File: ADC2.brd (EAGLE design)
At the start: 99.1 x 88.9 mm, 166 parts, among them IC1 FPGA CORE BOARD, IC10 AK1110, IC11 AD4001, IC12 TAR5SB33, IC13 74HC3G34, IC14 TC7WH74FU, IC15 NJM12888F18, IC16 TAR5SB33, IC2 OPA, IC3 OPA-DIFF, IC4 DCDC2, IC5 OPA-DIFF, IC6 OPA-DIFF, IC7 LM317-L, IC8 LM337-L, IC9 LM337-L, J1 DC, J10 ADC+, J11 GND, J12 ADC-, J2 DC, J3 VCOM, J4 GND, J5 VCOM, J6 V-, J7 V-, J8 V-, J9 V-, X1 12MHz

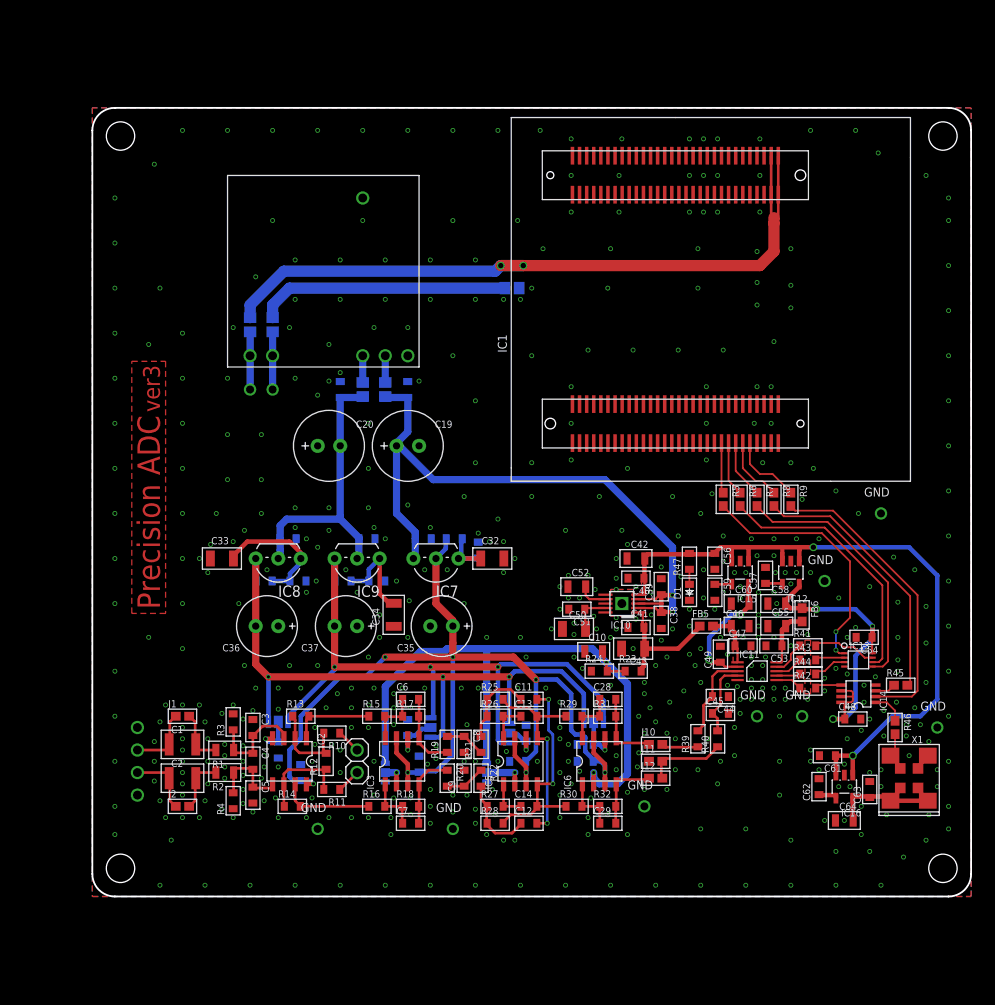
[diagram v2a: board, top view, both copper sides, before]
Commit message: AD4134
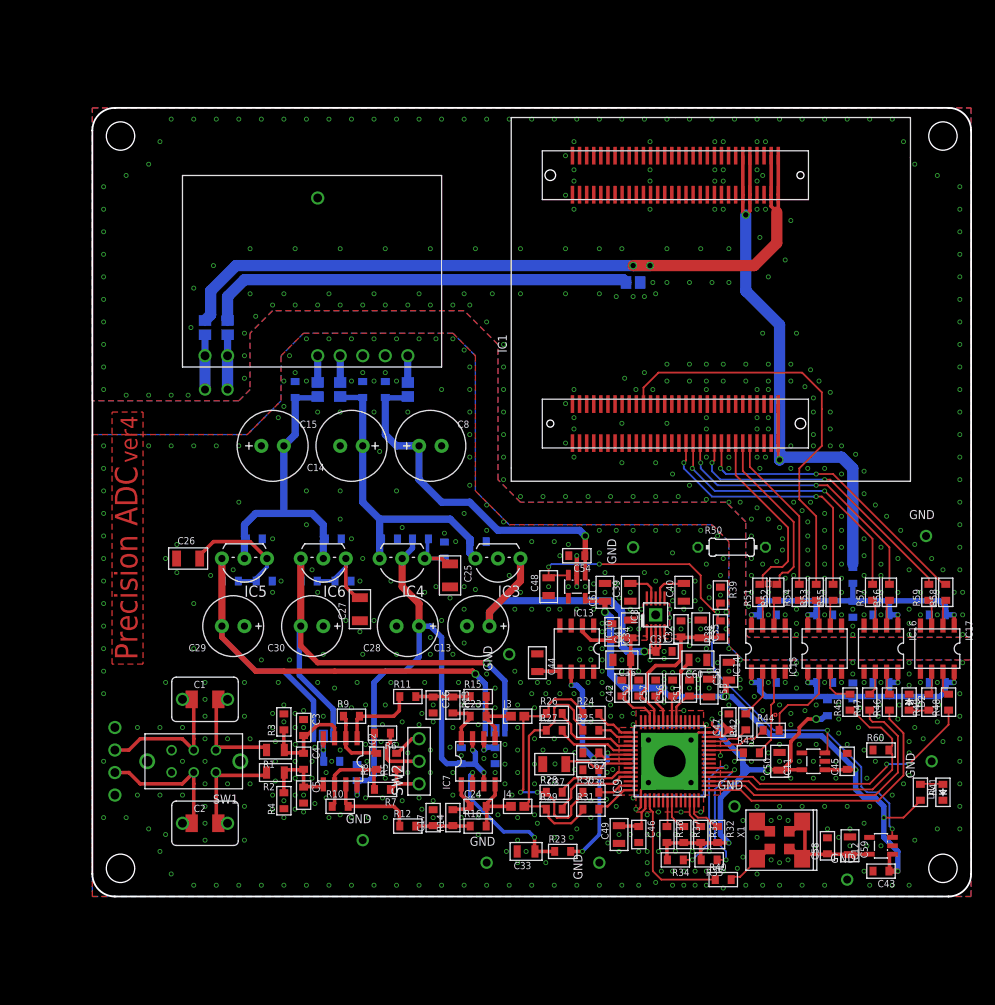
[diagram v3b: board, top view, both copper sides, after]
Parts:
- removed J10: ADC+, my_rcl:1608-J
- removed J11: GND, my_rcl:1608-J
- removed J12: ADC-, my_rcl:1608-J
- removed J5: VCOM, my_rcl:1608-3-J
- removed J6, J7, J8, J9: V-, my_rcl:2012-3-J
- removed JP1: GAIN, my_connector:1X02
- added C65, C66, C67, C68, C69, C70, C71: 0.1u, my_rcl:1608C
- added C72: 10u, my_rcl:1608C
- added D2: LED, my_rcl:D1608
- added FB7, FB8: FB, my_rcl:1608-FB
- added IC17: IOS6720FB, my_ic:SOP8
- added R48, R58: SDI, my_rcl:1608
- added R49, R59: LED, my_rcl:1608
- added R50: 10M, my_rcl:0204/7
- added R51: ODR, my_rcl:1608
- added R52: DOUT, my_rcl:1608
- added R53: SUB, my_rcl:1608
- added R54: DCLK, my_rcl:1608
- added R55: SDO, my_rcl:1608
- added R56: CS, my_rcl:1608
- added R57: SCLK, my_rcl:1608
- added R60: 10k, my_rcl:1608
- added SW1: DC, my_connector:SS22E01G5
- added SW2: GAIN, my_connector:1X03
- added TP13: GND, my_connector:TESTPIN
- added U1: DC-DC, my_ic:DCDC
- C1, C2: device my_rcl:3225 -> my_rcl:C050W
- C10: value 10u -> 1u; device my_rcl:2012 -> my_rcl:1608C
- C11, C12: value 1n -> 0.1u
- C13: value 1.5n -> 100u; device my_rcl:1608C -> my_rcl:E2.5-6.5
- C14: value 1.5n -> 100u; device my_rcl:1608C -> my_rcl:E2,5-8
- C15: value 1u -> 100u; device my_rcl:1608C -> my_rcl:E2,5-8
- C16: value 1u -> 1n
- C17: value 0.1u -> 1n
- C19, C20: value 100u -> 0.1u; device my_rcl:E2,5-8 -> my_rcl:1608C
- C23, C24: value 0.1u -> 270p
- C25, C26, C27: value 0.1u -> 10u; device my_rcl:1608C -> my_rcl:3216
- C28, C29: value 10p -> 100u; device my_rcl:1608C -> my_rcl:E2.5-6.5
- C30: value 0.1u -> 100u; device my_rcl:1608C -> my_rcl:E2.5-6.5
- C31, C62: value 0.1u -> 1u
- C32, C34: value 10u -> 1u; device my_rcl:3216 -> my_rcl:1608C
- C33, C50: device my_rcl:3216 -> my_rcl:2012
- C35, C36: value 100u -> 10u; device my_rcl:E2.5-6.5 -> my_rcl:2012
- C37: value 100u -> 10u; device my_rcl:E2.5-6.5 -> my_rcl:3216
- C38: value 1u -> 0.1u
- C39, C40, C41: value 1u -> 10u; device my_rcl:1608C -> my_rcl:2012
- C42, C46, C52, C58, C64: value 10u -> 0.1u; device my_rcl:2012 -> my_rcl:1608C
- C43: value 10u -> 0.1u; device my_rcl:3216 -> my_rcl:1608C
- C44: value 470p -> 10u; device my_rcl:1608C -> my_rcl:2012
- C45: value 470p -> 0.1u
- C47: value 3300p -> 0.1u
- C48, C49, C53, C59, C61: value 0.1u -> 10u; device my_rcl:1608C -> my_rcl:2012
- C51: value DNP -> 0.1u
- C6: value 10p -> 0.1u
- C63: value 0.1u -> 10u
- C7: value 10p -> 1u
- C8: value 2.7n -> 100u; device my_rcl:1608C -> my_rcl:E2,5-8
- C9: value 2.7n -> 1u
- FB5, FB6: device my_rcl:1608-J -> my_rcl:2012-J
- IC10: value AK1110 -> REF5040; device my_ic:PLP10 -> my_ic:SOP8
- IC11: value AD4001 -> 1.8V; device my_ic:MSOP10 -> my_ic:SOT23-5
- IC12: value TAR5SB33 -> 1.8V
- IC13: value 74HC3G34 -> 2.7V; device my_ic:SOT765 -> my_ic:SOT23-5
- IC14: value TC7WH74FU -> ISO6720FB; device my_ic:SSOP8-P-0.65 -> my_ic:SOP8
- IC15: value NJM12888F18 -> ISO6720FB; device my_ic:SOT23-5 -> my_ic:SOP8
- IC16: value TAR5SB33 -> IOS6720FB; device my_ic:SOT23-5 -> my_ic:SOP8
- IC3: value OPA-DIFF -> 7808; device my_ic:SOP8 -> my_ic:TO-92
- IC4: value DCDC2 -> LM317-L; device my_ic:DCDC2 -> my_ic:TO-92
- IC5, IC6: value OPA-DIFF -> LM337-L; device my_ic:SOP8 -> my_ic:TO-92
- IC7: value LM317-L -> OPA1633; device my_ic:TO-92 -> my_ic:SOP8
- IC8: value LM337-L -> AK1110; device my_ic:TO-92 -> my_ic:PLP10
- IC9: value LM337-L -> AD4134; device my_ic:TO-92 -> my_ic:QFN56-HT-HOLE
- J1, J2: value DC -> V-; device my_rcl:1608-J -> my_rcl:2012-3-J
- J3: value VCOM -> ADC+; device my_rcl:1608-3-J -> my_rcl:1608-J
- J4: value GND -> ADC-; device my_rcl:2012-J -> my_rcl:1608-J
- R10, R11: value 100 -> 1k
- R13, R14: value 1k -> 360
- R17, R18: value 1k -> 680
- R19: value 1k -> 330
- R20, R21, R22, R23: value 1k -> 120
- R24, R26, R27, R29, R30, R31: value 1k -> 22
- R25, R28: value 3.6k -> 22
- R3, R4: value 10k -> 100k
- R32: value 1k -> 10k
- R33, R34: value 680 -> 10k
- R35: value 330 -> 10k
- R36, R37: value 120 -> 10k
- R38: value 120 -> 47k
- R39: value 22 -> 47k
- R40: value 22 -> 39
- R41: value 37 -> 5.1k
- R42: value 37 -> ODR
- R43: value 37 -> DOUT
- R44: value 37 -> DCLK
- R45: value 37 -> SDO; device my_rcl:1608-J -> my_rcl:1608
- R46: value 37 -> CS; device my_rcl:1608-J -> my_rcl:1608
- R47: value 5.1k -> SCLK
- R5: value 22 -> 360; device my_rcl:1608-J -> my_rcl:1608
- R6, R7: value 22 -> 10; device my_rcl:1608-J -> my_rcl:1608
- R8: value 22 -> 10k; device my_rcl:1608-J -> my_rcl:1608
- R9: value 22 -> 1k; device my_rcl:1608-J -> my_rcl:1608
- X1: value 12MHz -> 48MHz
- moved FB6 60.2 mm to (25.4, 57.1), flipped to the bottom
- moved J4 58.4 mm to (47.9, 10.2), flipped to the top
- moved R37 55.3 mm to (66.7, 6.99), flipped to the top, turned to 270 degrees
- moved R9 55.2 mm to (29.2, 20.3), turned to 0 degrees
- moved R8 53.6 mm to (32.1, 15.2), turned to 90 degrees
- moved R7 53.4 mm to (32.7, 12.1), turned to 180 degrees
- moved R34 52.9 mm to (65.7, 4.13), flipped to the top
- moved FB5 49.1 mm to (27.9, 57.1), flipped to the bottom, turned to 270 degrees
- moved C7 49.0 mm to (33.0, 57.1), flipped to the bottom, turned to 90 degrees
- moved R35 48.9 mm to (69.5, 4.13), flipped to the top
- moved R6 48.2 mm to (32.7, 18.4), turned to 180 degrees
- moved C29 47.7 mm to (15.9, 30.5), turned to 180 degrees
- moved C33 47.6 mm to (48.9, 5.08)
- moved R5 47.2 mm to (34.3, 15.2), turned to 90 degrees
- moved C14 45.3 mm to (29.2, 50.8), turned to 180 degrees
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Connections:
- removed net +3V3A: C48.1, C54.1, C58.1, FB6.1, IC12.5, IC13.8, IC14.6, IC14.7, IC14.8
- removed net ADC+_LPF: C44.2, IC11.3, R39.2
- removed net ADC-_LPF: C45.1, IC11.4, R40.2
- removed net ADC_CNVST: IC14.2, R9.2
- removed net ADC_CNVST_CLOCKED: IC14.5, R42.2
- removed net ADC_CNVST_FB: R45.2, R8.2
- removed net ADC_SCK: IC13.6, R6.2
- removed net CLK_8MHZ: R46.2, X1.3, X1.3-2
- removed net N$57: FB2.1, J4.2
- new net +1V8_ISO: C63.1, C64.1, C65.1, C66.1, C67.1, FB7.2, IC14.1, IC15.1, IC16.8, IC17.8
- new net +3.6V: C54.1, C7.1, C8.+, FB4.1, IC13.1
- new net +3V3D: FB8.2, IC1.109, IC1.110, IC1.111, IC1.112, IC1.59, IC1.60
- new net +3V3D_ISO: C68.1, C69.1, C70.1, C71.1, C72.1, FB8.1, IC14.8, IC15.8, IC16.1, IC17.1
- new net +5V_DEL: C48.1, IC11.3, IC12.3, IC13.3, R38.2, R39.2
- new net +8V: C13.+, C31.1, IC3.1, IC8.2, IC8.3, IC8.4
- new net ADC_2V7: C43.1, C45.1, C55.1, C57.1, C61.1, IC11.1, IC12.1, IC13.5, IC9.23, R41.2
- new net ADC_AVDD1V8: C56.1, C60.1, IC9.21
- new net ADC_CLKVDD: C46.1, C49.1, IC9.44
- new net ADC_CS: IC9.1, R46.1
- new net ADC_DCLK: IC9.11, R44.1
- new net ADC_DOUT: IC9.10, R43.1
- new net ADC_DVDD1V8: C51.1, C53.1, IC9.20
- new net ADC_ODR: IC9.12, R42.1
- new net ADC_SCLK: IC9.2, R47.1
- new net AVDD5V: C34.1, C36.1, C41.1, C42.1, IC10.2, IC8.1, IC9.26
- new net DGND: C68.2, C69.2, C70.2, C71.2, C72.2, FB1.1, IC1.1, IC1.101, IC1.102, IC1.103, IC1.104, IC1.113, IC1.114, IC1.115, IC1.116, IC1.2, IC1.39, IC1.40, IC1.53, IC1.54, IC1.57, IC1.58, IC1.61, IC1.62, IC1.83, IC1.84, IC14.5, IC15.5, IC16.4, IC17.4, R50.2, TP13.1
- new net FPGA_CS: IC1.38, R56.2
- new net FPGA_DCLK: IC1.52, R54.2
- new net FPGA_DCLK_SUB: IC1.21, R53.2
- new net FPGA_DOUT: IC1.50, R52.2
- new net FPGA_LED: IC1.42, R59.2
- new net FPGA_ODR: IC1.48, R51.2
- new net FPGA_SCLK: IC1.36, R57.2
- new net FPGA_SDI: IC1.44, R58.2
- new net FPGA_SDO: IC1.34, R55.2
- new net N$60: IC9.50, R37.1
- new net N$61: IC9.55, R32.1
- new net N$62: IC9.54, R33.1
- new net N$64: IC9.49, R36.1
- new net OSC_CLK: IC9.45, R40.1
- new net VREFCAP: C37.1, C38.1, IC9.36
- net +1V8: now also C47.1, C50.1, FB7.1, IC11.5, IC9.13, R32.2, R33.2, R34.2, R35.2, R36.2, R37.2; no longer C49.1, C60.1, IC11.2, IC15.5
- net +5V: now also C32.1, C35.1, C52.1, IC8.5, IC9.25, R38.1; no longer C40.1, C42.1, C56.1, C61.1, IC10.5, IC12.1, IC12.3, IC15.1, IC15.3, IC16.1, IC16.3, R47.2
- net +9V: now also C11.1, C28.+, IC4.2, IC7.3, IC7.7, R20.2; no longer C17.1, C26.1, C30.1, C35.+, IC3.3, IC3.7, IC5.3, IC5.7, IC6.3, IC6.7, IC7.2, R36.2
- net -5V: now also C30.-, IC6.3, J1.1, J2.1, R22.2; no longer C37.-, IC9.3, J6.1, J7.1, J8.1, J9.1, R38.2
- net -9V: now also C29.-, IC5.3, J1.3, J2.3, R21.2; no longer C36.-, IC8.3, J6.3, J7.3, J8.3, J9.3, R37.2
- net ADC+: now also J3.2, R24.1, R26.1, R28.1, R30.1; no longer J10.2, R39.1
- net ADC-: now also J4.2, R25.1, R27.1, R29.1, R31.1; no longer J11.2, J12.2, R40.1
- net ADC_SDI: now also IC9.4, R48.1; no longer IC13.1, R5.2
- net ADC_SDO: now also IC9.3, R45.1, R60.2; no longer IC13.5, R7.2
- net ADC_VCOM: now also C33.2, IC7.2; no longer C10.1, IC6.2, J3.3, J5.3, R24.2
- net GND: now also C10.1, C11.2, C12.1, C13.-, C14.-, C15.+, C16.2, C18.2, C19.1, C20.1, C25.2, C26.1, C28.-, C29.+, C30.+, C31.2, C34.2, C35.2, C36.2, C37.2, C44.2, C6.2, C65.2, C66.2, C67.2, C7.2, C8.-, D2.K, IC10.4, IC11.2, IC13.2, IC15.4, IC16.5, IC17.5, IC3.2, IC8.10, IC8.6, IC8.8, IC8.HT, IC9.14, IC9.19, IC9.22, IC9.24, IC9.27, IC9.31, IC9.37, IC9.40, IC9.43, IC9.47, IC9.HT, IC9.HT1, IC9.HT2, IC9.HT3, IC9.HT4, R17.1, R18.2, R19.2, R39.1, R50.1, R60.1, SW1.HT1, SW1.HT2, U1.GND1, U1.GND2; no longer C10.2, C15.2, C16.1, C18.1, C19.-, C20.+, C23.2, C24.1, C25.1, C26.2, C30.2, C31.1, C34.1, C35.-, C36.+, C37.+, C44.1, C8.2, IC1.1, IC1.101, IC1.102, IC1.103, IC1.104, IC1.113, IC1.114, IC1.115, IC1.116, IC1.2, IC1.39, IC1.40, IC1.53, IC1.54, IC1.57, IC1.58, IC1.61, IC1.62, IC1.83, IC1.84, IC10.10, IC10.6, IC10.8, IC10.HT, IC11.5, IC13.4, IC15.2, IC16.2, IC4.GND1, J11.1, J3.1, J4.1, J5.1, R24.1, R33.1, R34.2, R35.2
- net N$1: now also R10.1, R7.2, R8.1; no longer R11.2, R12.1, R14.1
- net N$10: now also IC15.2, R44.2; no longer IC1.46, R6.1
- net N$11: now also IC9.42, R31.2; no longer IC14.3, R45.1
- net N$12: now also R10.2, R12.1; no longer R14.2, R16.1
- net N$13: now also IC9.41, R30.2; no longer IC13.7, R41.2
- net N$15: now also IC9.39, R29.2; no longer C53.1, C55.1, FB6.2, IC11.10
- net N$16: now also IC15.3, R45.2; no longer C46.1, C47.1, FB5.2, IC11.1
- net N$17: now also IC14.6, R52.1; no longer IC1.48, R7.1
- net N$18: now also IC9.38, R28.2; no longer IC14.1, R46.1
- net N$19: now also C17.1, R12.2, R14.1, R16.1; no longer C29.1, IC6.1, R30.2, R32.1
- net N$2: now also IC9.34, R23.2; no longer C29.2, IC6.4, J12.1, R32.2
- net N$20: now also IC9.33, R27.2; no longer IC13.3, R44.2
- net N$21: now also IC14.7, R51.1; no longer IC1.52, R9.1
- net N$22: now also C23.2, IC7.5, J3.1, R15.2; no longer C28.1, IC6.8, R29.2, R31.1
- net N$24: now also C23.1, IC7.8, R13.2; no longer C8.1, R19.2, R21.1
- net N$25: now also IC9.32, R26.2; no longer IC11.7, R44.1
- net N$26: now also C24.1, IC7.1, R14.2; no longer C9.1, R20.2, R22.1
- net N$27: now also IC15.7, R53.1, R54.1; no longer C13.1, IC5.8, R26.2
- net N$28: now also IC9.30, R25.2; no longer IC11.8, R43.1
- net N$29: now also IC9.29, R24.2; no longer IC11.6, R42.1
- net N$3: now also R6.2, R8.2, R9.1; no longer R10.2, R12.2, R13.1
- net N$30: now also R40.2, X1.3, X1.3-2; no longer IC11.9, R41.1
- net N$31: now also C24.2, IC7.4, J4.1, R16.2; no longer IC13.2, R43.2
- net N$32: now also IC15.6, R55.1; no longer C12.2, C13.2, IC5.5, R25.2, R29.1
- net N$33: now also IC16.6, R47.2; no longer C11.2, C14.2, IC5.4, R28.2, R30.1
- net N$34: now also IC16.7, R46.2; no longer C14.1, IC5.1, R27.2
- net N$35: now also IC17.6, R49.2; no longer C12.1, R22.2, R27.1, R28.1
- net N$36: now also IC17.7, R48.2; no longer C11.1, R21.2, R25.1, R26.1
- net N$37: now also IC16.3, R57.1; no longer C7.2, IC3.4, R18.2, R20.1
- net N$38: now also IC16.2, R56.1; no longer C6.2, IC3.5, R17.2, R19.1
- net N$39: now also IC17.3, R59.1; no longer C7.1, IC3.1, R16.2, R18.1
- net N$4: now also R11.1, R9.2; no longer R13.2, R15.1
- net N$40: now also IC17.2, R58.1; no longer C6.1, IC3.8, R15.2, R17.1
- net N$41: now also C1.3, SW1.C2; no longer J1.1
- net N$42: now also C2.3, SW1.C1; no longer J2.1
- net N$43: now also C1.4, SW1.A2; no longer J1.2
- net N$44: now also C2.4, SW1.A1; no longer J2.2
- net N$45: now also R6.1, SW2.2; no longer JP1.1, R10.1
- net N$46: now also R5.1, R7.1, SW2.1; no longer JP1.2, R11.1
- net N$47: now also D2.A, R49.1; no longer IC5.2, J5.2
- net N$48: now also C44.1, IC10.5; no longer C62.1, IC16.4
- net N$49: now also IC9.5, R35.1; no longer IC3.2, J3.2
- net N$5: now also C16.1, R11.2, R13.1, R15.1; no longer C28.2, IC6.5, J10.1, R31.2
- net N$50: now also IC9.6, R34.1; no longer C27.2, IC5.6, J8.2
- net N$51: now also FB4.2, U1.+5V; no longer C22.2, IC3.6, J7.2
- net N$52: now also C12.2, J1.2; no longer C18.2, J6.2
- net N$53: now also C25.1, IC4.1, R17.2, R20.1; no longer C32.1, IC7.1, R33.2, R36.1
- net N$54: now also C26.2, IC5.1, R18.1, R21.1; no longer C33.2, IC8.1, R34.1, R37.1
- net N$55: now also C27.2, IC6.1, R19.1, R22.1; no longer C34.2, IC9.1, R35.1, R38.1
- net N$56: now also FB1.2, FB3.1; no longer C57.1, IC12.4
- net N$58: now also R41.1; no longer R47.1
- net N$59: now also R5.2, SW2.3; no longer C59.1, IC15.4
- net N$6: now also C39.1, IC8.9; no longer IC1.50, R8.1
- net N$7: now also C40.1, IC8.7; no longer C52.1, IC10.7
- net N$70: now also FB5.1, U1.V+; no longer FB3.1, IC4.V+
- net N$71: now also FB6.1, U1.V-; no longer FB4.1, IC4.V-
- net N$74: now also C22.2, IC7.6, J2.2; no longer C31.2, IC6.6, J9.2
- net N$75: now also FB2.2, U1.VIN+; no longer FB1.2, IC4.VIN+
- net N$76: now also FB3.2, U1.VIN-; no longer FB2.2, IC4.VIN-
- net N$8: now also IC14.2, R42.2; no longer C50.1, C51.1, IC10.9
- net N$9: now also IC14.3, R43.2; no longer IC1.44, R5.1
- net V+: now also C14.+, C18.1, C6.1, C9.1, FB5.2, IC3.3, IC4.3; no longer C15.1, C19.+, C23.1, C38.1, C39.1, FB3.2, IC10.2, IC10.3, IC10.4, IC7.3
- net V-: now also C10.2, C15.-, C19.2, C20.2, FB6.2, IC5.2, IC6.2; no longer C16.2, C20.-, C24.2, C25.2, FB4.2, IC8.2, IC9.2
- net VCC_OSC: now also C58.1, C59.1, IC12.5; no longer C63.1, C64.1, IC16.5
- net VIN: now also FB2.1; no longer FB1.1
- net VREF: now also C62.1, IC10.6, IC9.35; no longer C41.1, C43.1, FB5.1, IC10.1, R23.2
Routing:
- net ADC_2V7: track 0.00 -> 75.8 mm, vias 0 -> 6
- net +5V_DEL: track 0.00 -> 69.8 mm, vias 0 -> 5
- net +3V3D: track 0.00 -> 69.3 mm, vias 0 -> 2
- net +5V: track 81.1 -> 18.3 mm, vias 2 -> 0
- net ADC_VCOM: track 73.4 -> 17.3 mm
- net +9V: track 117.3 -> 62.9 mm, vias 7 -> 3
- net FPGA_DCLK_SUB: track 0.00 -> 47.1 mm
- net N$56: track 1.94 -> 48.5 mm
- net V+: track 78.2 -> 35.3 mm, vias 2 -> 0
- net +8V: track 0.00 -> 41.9 mm, vias 0 -> 1
- net +3.6V: track 0.00 -> 40.8 mm, vias 0 -> 1
- net +3V3A: track 38.0 -> 0.00 mm, vias 3 -> 0
- net +3V3D_ISO: track 0.00 -> 37.6 mm, vias 0 -> 4
- net +1V8_ISO: track 0.00 -> 36.1 mm, vias 0 -> 4
- net ADC_CNVST: track 34.3 -> 0.00 mm
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- added copper zone on layer 1, net AVDD5V
- added copper zone on layer 1, net DGND
- added copper zone on layer 15, net DGND
- added copper zone on layer 16, net DGND
- added copper zone on layer 2, net DGND
- removed copper zone on layer 1, net N$16
- removed copper zone on layer 1, net VREF
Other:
- board text added: "ver4"
- board text removed: "ver3"

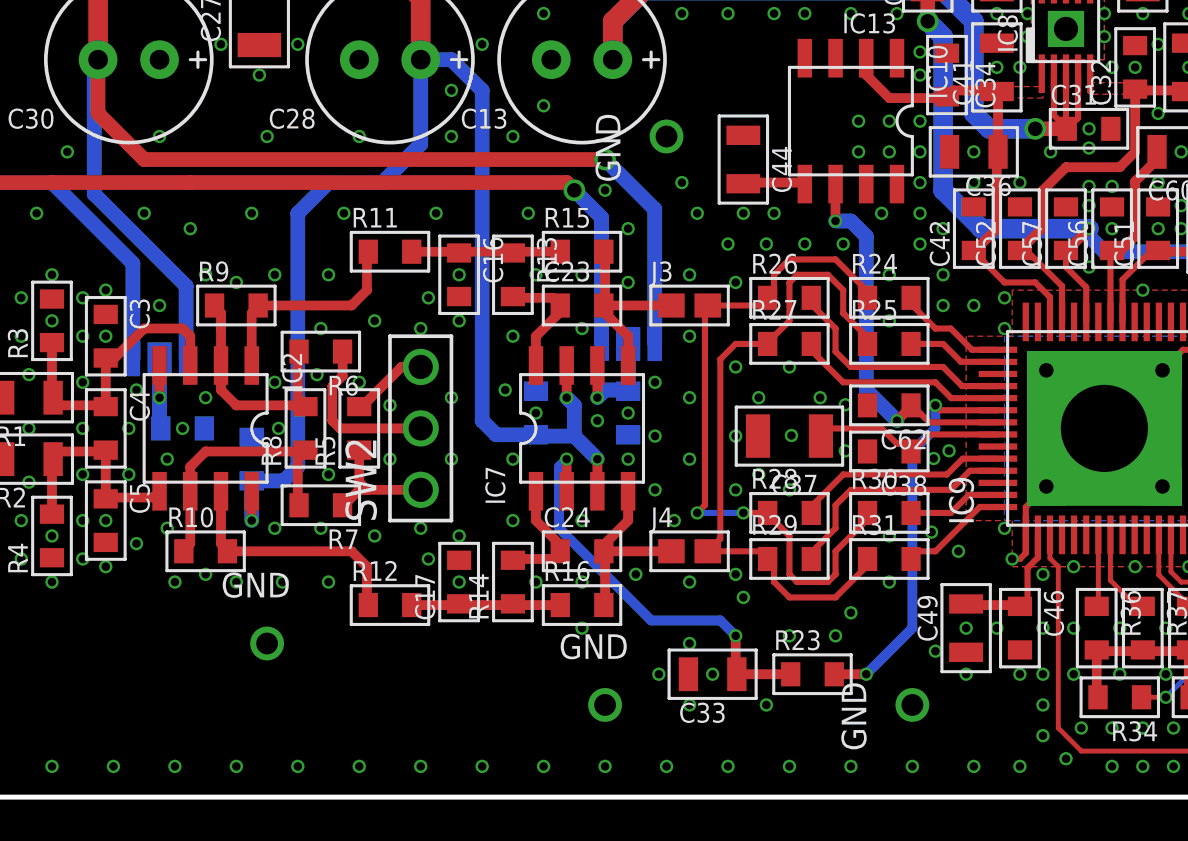
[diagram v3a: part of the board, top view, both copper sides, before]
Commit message: 発注
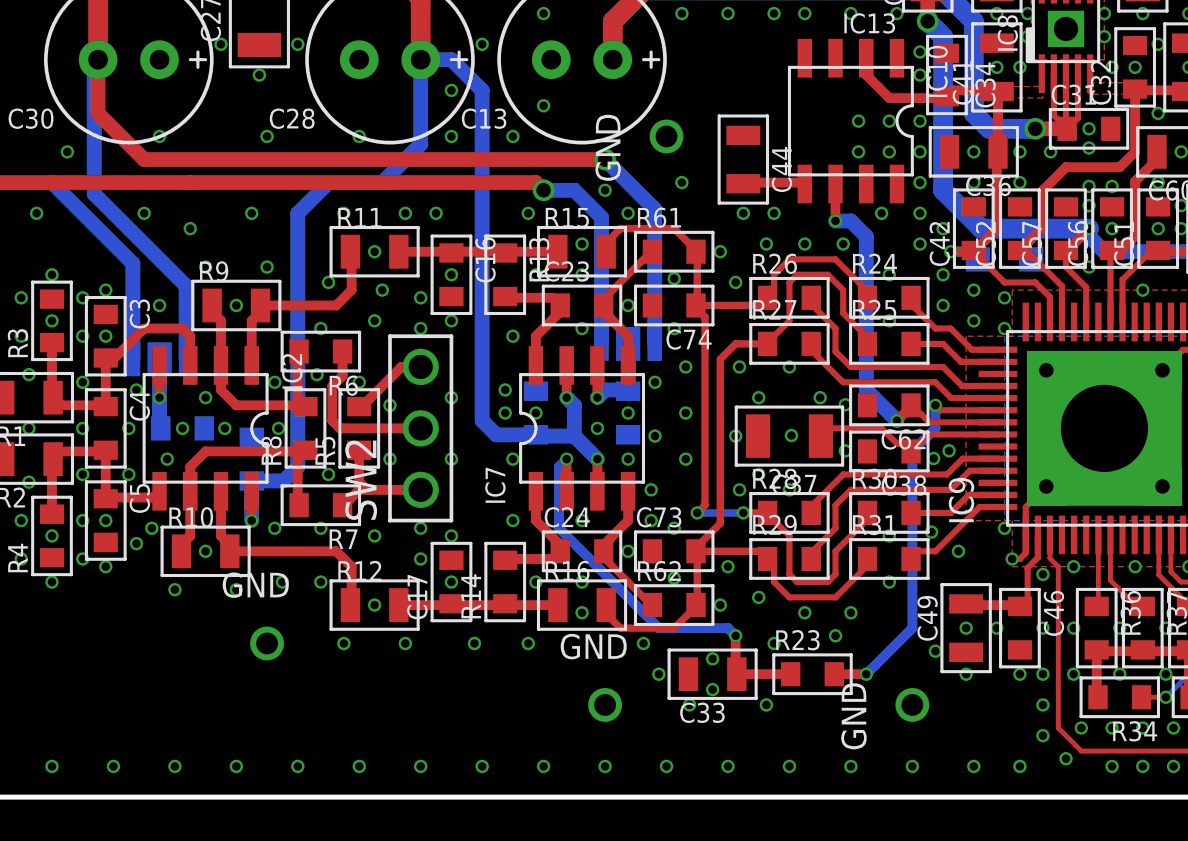
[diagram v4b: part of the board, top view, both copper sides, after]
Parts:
- removed J3: ADC+, my_rcl:1608-J
- removed J4: ADC-, my_rcl:1608-J
- added C73, C74: 47p, my_rcl:1608C
- added D3: TVS, my_rcl:SOD323
- added R61, R62: 50, my_rcl:1608
- R10, R11, R12, R15, R16, R9: device my_rcl:1608 -> my_rcl:2012
- moved R11 0.64 mm to (34.9, 22.5)
- moved R12 0.64 mm to (34.9, 7.94)
- moved R13 0.32 mm to (40.3, 21.6)
- moved R14 0.32 mm to (40.3, 8.89)
- moved C16 0.32 mm to (38.1, 21.6)
- moved C17 0.32 mm to (38.1, 8.89)
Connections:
- net ADC+: now also C74.1, R15.2, R61.2; no longer J3.2
- net ADC-: now also C73.2, R16.2, R62.2; no longer J4.2
- net AVDD5V: now also D3.2
- net GND: now also C73.1, C74.2, D3.1
- net N$22: now also R61.1; no longer J3.1, R15.2
- net N$31: now also R62.1; no longer J4.1, R16.2
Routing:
- net ADC-: track 27.2 -> 34.8 mm
- net ADC+: track 28.4 -> 36.0 mm
- net AVDD5V: track 18.7 -> 21.7 mm, vias 0 -> 1
- net N$22: track 7.96 -> 5.98 mm
- net N$31: track 7.91 -> 6.01 mm
- net N$12: track 10.2 -> 9.53 mm
- net N$4: track 8.96 -> 8.29 mm
- net GND: vias 539 -> 556
